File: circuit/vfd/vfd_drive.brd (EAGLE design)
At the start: 100 x 100 mm, 41 parts, among them J1 ZX62R-AB-5P, J3 FSM-21045-7, J5 PSM-210223-7, J7 DC_JACK_2DC0005D100, Q1 BSS138, Q2 BSS138, U1 CP2104, U2 MAX6921AWI+, U3 NJM2360AM, U5 ADP3338AKCZ-3.3, U6 RX8035LC, U8 ESP-WROOM-32

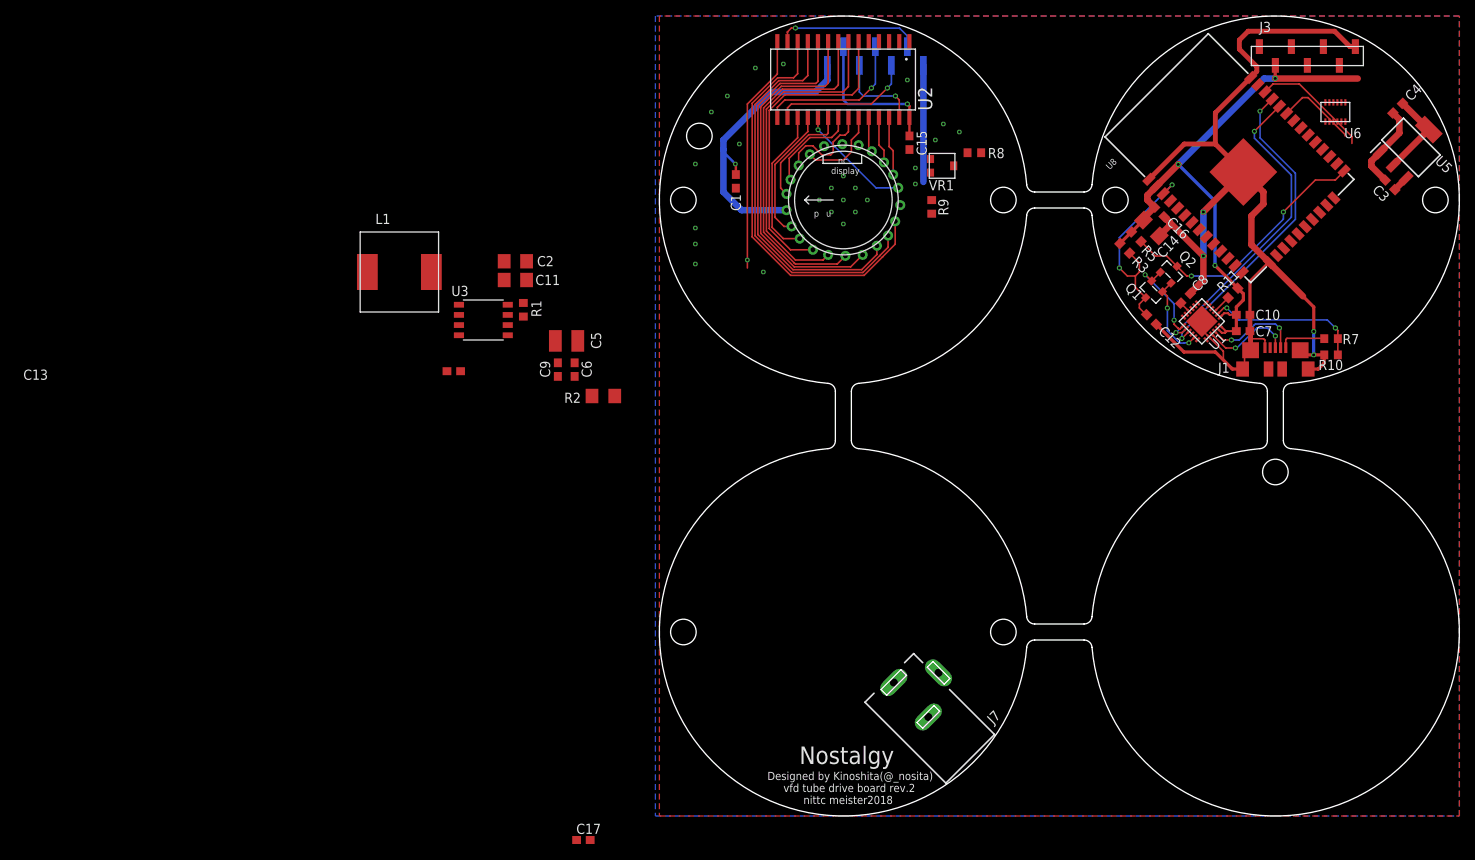
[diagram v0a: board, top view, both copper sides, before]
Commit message: [add]add all
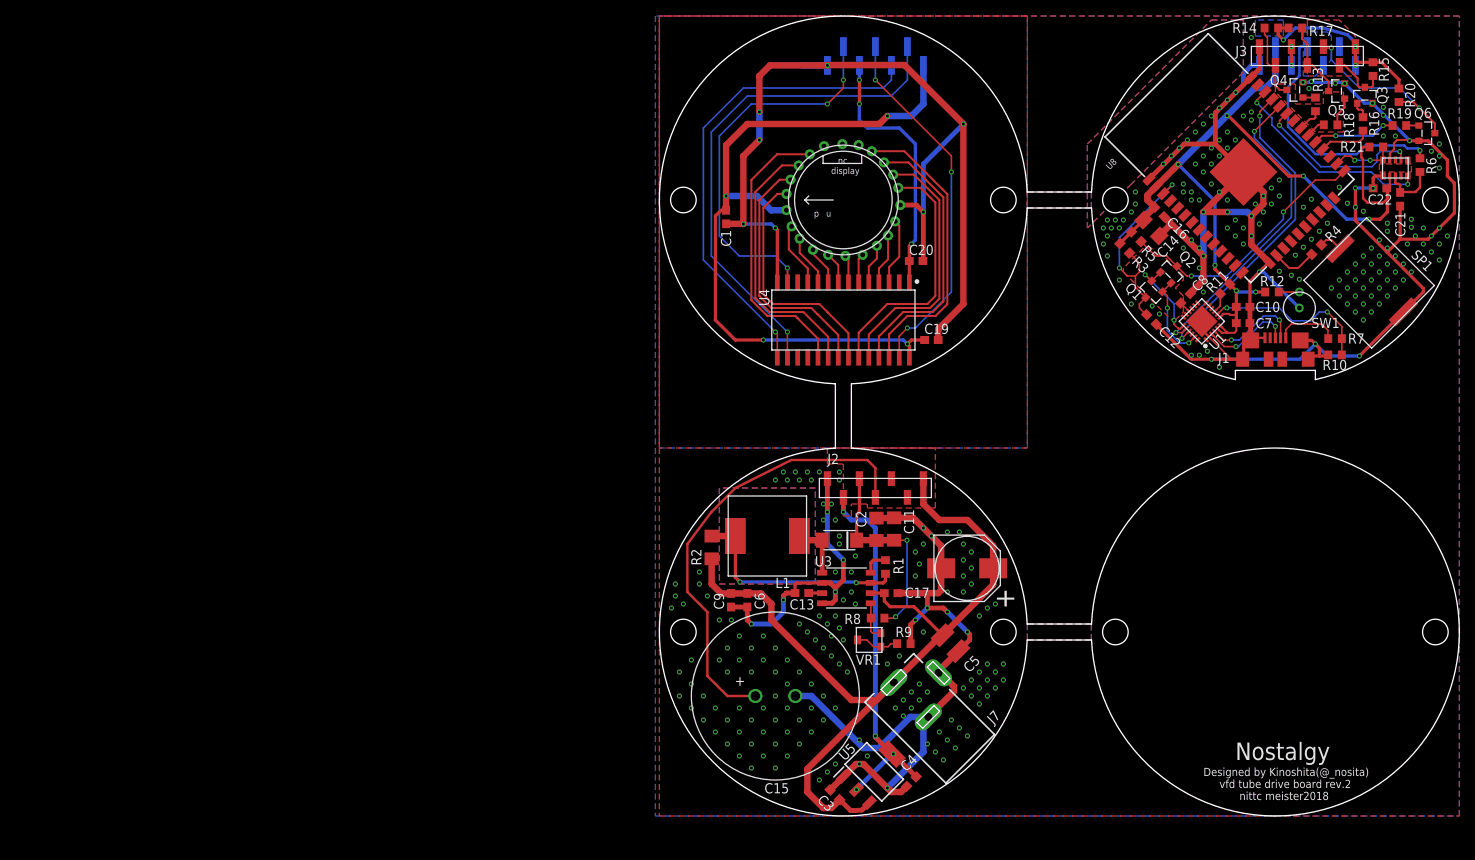
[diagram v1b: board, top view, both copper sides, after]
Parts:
- removed U6: RX8035LC, taki-library:VSOJ12
- added C18: UWT1E221MNL1GS, taki-library:NICHICON-ALMINUM-CAPACITOR-8MM
- added C19, C20, C21, C22: 0.1uF, taki-library:C0603
- added D1: MS18F, taki-library:SMAF
- added J2: FSM-21045-7, taki-library:FSM-21045-7
- added J4: PSM-210223-7, taki-library:PSM-210223-7
- added Q3, Q4, Q5, Q6: BSS138, taki-library:SOT23-N-MOSFET
- added R12, R14, R15, R17, R20, R21, R4, R6: 10k, taki-library:R0603
- added R13, R16, R18, R19: 1k, taki-library:R0603
- added SP1: PKLCS1212E4001-R1, taki-library:PKLCS1212E4001-R1
- added SW1: AT407, taki-library:AT407
- added U4: HV5812SOW, taki-library:SOW28-MICROCHIP
- C13: value 680pF -> 470pF
- C15: value 0.1uF -> (none); device taki-library:C0603 -> taki-library:SE-5R5-D155VY
- R2: value 0.02 -> 0.2
- R8: value 3.3k -> 220k
- R9: value 3.3k -> 8.2k
- U2: value MAX6921AWI+ -> RX8900CE; device taki-library:SOIC-28-MI -> taki-library:RX8900CE
- moved C4 103.8 mm to (31.5, 4.29)
- moved C3 103.1 mm to (21.9, 2.65)
- moved U5 102.9 mm to (26.9, 5.52)
- moved C15 71.2 mm to (14.5, 15.0), turned to 0 degrees
- moved U2 61.7 mm to (92.0, 81.0), turned to 0 degrees
- moved C5 61.1 mm to (36.4, 21.6), turned to 315 degrees
- moved VR1 60.0 mm to (26.2, 22.0), turned to 90 degrees
- moved R8 59.4 mm to (27.3, 24.7)
- moved C11 56.7 mm to (29.3, 35.9), turned to 90 degrees
- moved L1 56.6 mm to (13.5, 35.0)
- moved U3 56.4 mm to (23.4, 28.5)
- moved C2 56.2 mm to (27.1, 35.8), turned to 90 degrees
- moved R1 55.5 mm to (28.3, 31.1)
- moved R9 54.7 mm to (30.6, 21.5), turned to 180 degrees
- moved C13 51.6 mm to (17.8, 27.9)
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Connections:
- removed net N$18: J5.6, U2.13
- removed net VFBLANK: J3.6
- removed net VFCLK: J3.4
- removed net VFDIN: J3.3
- removed net VFLOAD: J3.5
- new net BATT: J4.4, R6.2
- new net BL: J5.2, U4.13
- new net CLK: J5.5, U4.15
- new net DATA: J5.4, U4.27
- new net EDLC: C15.POS, J2.4
- new net ESP32_BL: R13.2, U8.31
- new net ESP32_CLK: R19.2, U8.29
- new net ESP32_DATA: R18.2, U8.30
- new net ESP32_STR: R16.2, U8.28
- new net INT: R21.1, U2.10, U8.26
- new net N$10: R4.1, SP1.1
- new net N$15: Q5.G, R18.1
- new net SP: R4.2, U8.16
- new net STR: J5.6, U4.16
- new net SW: R12.1, SW1.1
- new net VFD_BL: J3.2, Q4.D, R14.1
- new net VFD_CLK: J3.5, Q6.D, R20.1
- new net VFD_DATA: J3.4, Q5.D, R17.1
- new net VFD_STR: J3.6, Q3.D, R15.1
- net +24V: now also C20.1, D1.K, J2.3, J3.3, J4.3, J5.3, U4.1; no longer U2.1
- net +3V3: now also C22.1, J2.2, J4.2, R12.2, R21.2, U2.2; no longer C15.1, J3.2, J5.2, U2.28, U6.2
- net +5V: now also C17.1, C18.POS, C19.1, J2.7, J3.7, J4.7, J5.7, R14.2, R15.2, R17.2, R20.2, U4.28; no longer J3.1, J5.1
- net GND: now also C15.NEG, C18.NEG, C19.2, C20.2, C21.2, C22.2, J2.1, J3.1, J4.1, J5.1, Q3.S, Q4.S, Q5.S, Q6.S, SP1.2, SW1.2, U2.1, U2.9, U4.14; no longer C15.2, J3.7, J5.7, U2.14
- net N$1: now also VR1.1, VR1.2; no longer VR1.3
- net N$12: now also VR1.3; no longer VR1.1, VR1.2
- net N$2: now also Q4.G, R13.1; no longer C17.1, U6.1
- net N$3: now also Q6.G, R19.1; no longer J5.3, U2.27
- net N$4: now also Q3.G, R16.1; no longer J5.4, U2.15
- net N$5: now also C21.1, R6.1, U2.3; no longer J5.5, U2.16
- net N$6: now also D1.A
- net SCL: now also U2.5; no longer U6.6
- net SDA: now also U2.7; no longer U6.8
- net VFD10: now also U4.20; no longer U2.22
- net VFD11: now also U4.21; no longer U2.21
- net VFD12: now also U4.22; no longer U2.20
- net VFD14: now also U4.11; no longer U2.18
- net VFD15: now also U4.10; no longer U2.17
- net VFD16: now also U4.9; no longer U2.6
- net VFD17: now also U4.8; no longer U2.7
- net VFD18: now also U4.7; no longer U2.8
- net VFD19: now also U4.6; no longer U2.9
- net VFD2: now also U4.23; no longer U2.19
- net VFD20: now also U4.5; no longer U2.10
- net VFD21: now also U4.4; no longer U2.11
- net VFD22: now also U4.3; no longer U2.12
- net VFD3: now also U4.24; no longer U2.26
- net VFD4: now also U4.25; no longer U2.25
- net VFD5: now also U4.26; no longer U2.24
- net VFD9: now also U4.19; no longer U2.23
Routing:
- net GND: track 208.1 -> 488.6 mm, vias 30 -> 327
- net +5V: track 39.0 -> 228.4 mm, vias 1 -> 7
- net STR: track 0.00 -> 63.5 mm, vias 0 -> 1
- net +24V: track 0.00 -> 63.2 mm, vias 0 -> 7
- net CLK: track 0.00 -> 60.3 mm, vias 0 -> 1
- net EDLC: track 0.00 -> 56.2 mm
- net +3V3: track 103.0 -> 157.2 mm, vias 4 -> 11
- net BL: track 0.00 -> 47.6 mm, vias 0 -> 3
- net DATA: track 0.00 -> 46.1 mm, vias 0 -> 3
- net VFD22: track 52.2 -> 8.37 mm
- net VFD21: track 50.0 -> 6.33 mm
- net VFD20: track 48.4 -> 5.01 mm
- net VFD19: track 45.7 -> 3.65 mm
- net VFD18: track 43.7 -> 3.47 mm
- net VFD17: track 41.7 -> 3.97 mm
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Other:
- outline, holes or cut-outs redrawn
